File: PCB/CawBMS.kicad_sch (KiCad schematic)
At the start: 37 parts, among them CN1 SWD, CN2 I2C, CN3 SPI, CN4 USART, CN5 SWD, SW1 B3U-1000P, SW2 B3U-1000P, U1 STM32F103CBTx, U2 TCAN1044DRBRQ1, U5 CAN, X1 Crystal_16MHz_15pF_3P

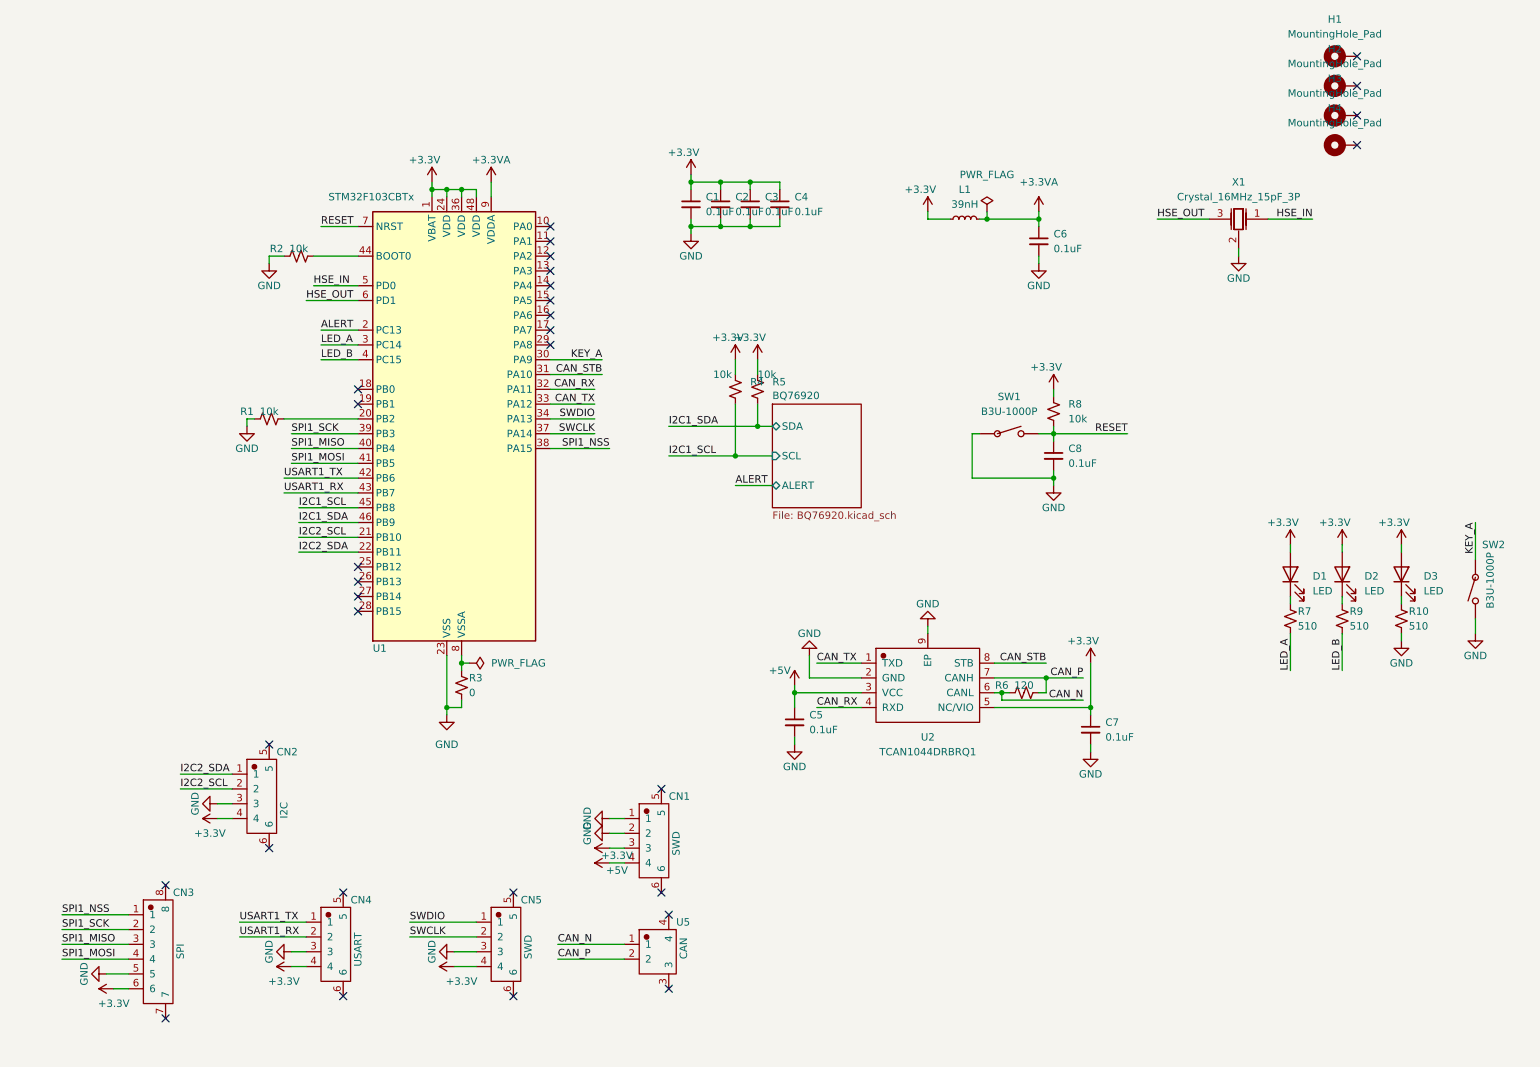
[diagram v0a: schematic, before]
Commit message: Signed-off-by: jasperThinkpad <2567434944@qq.com>
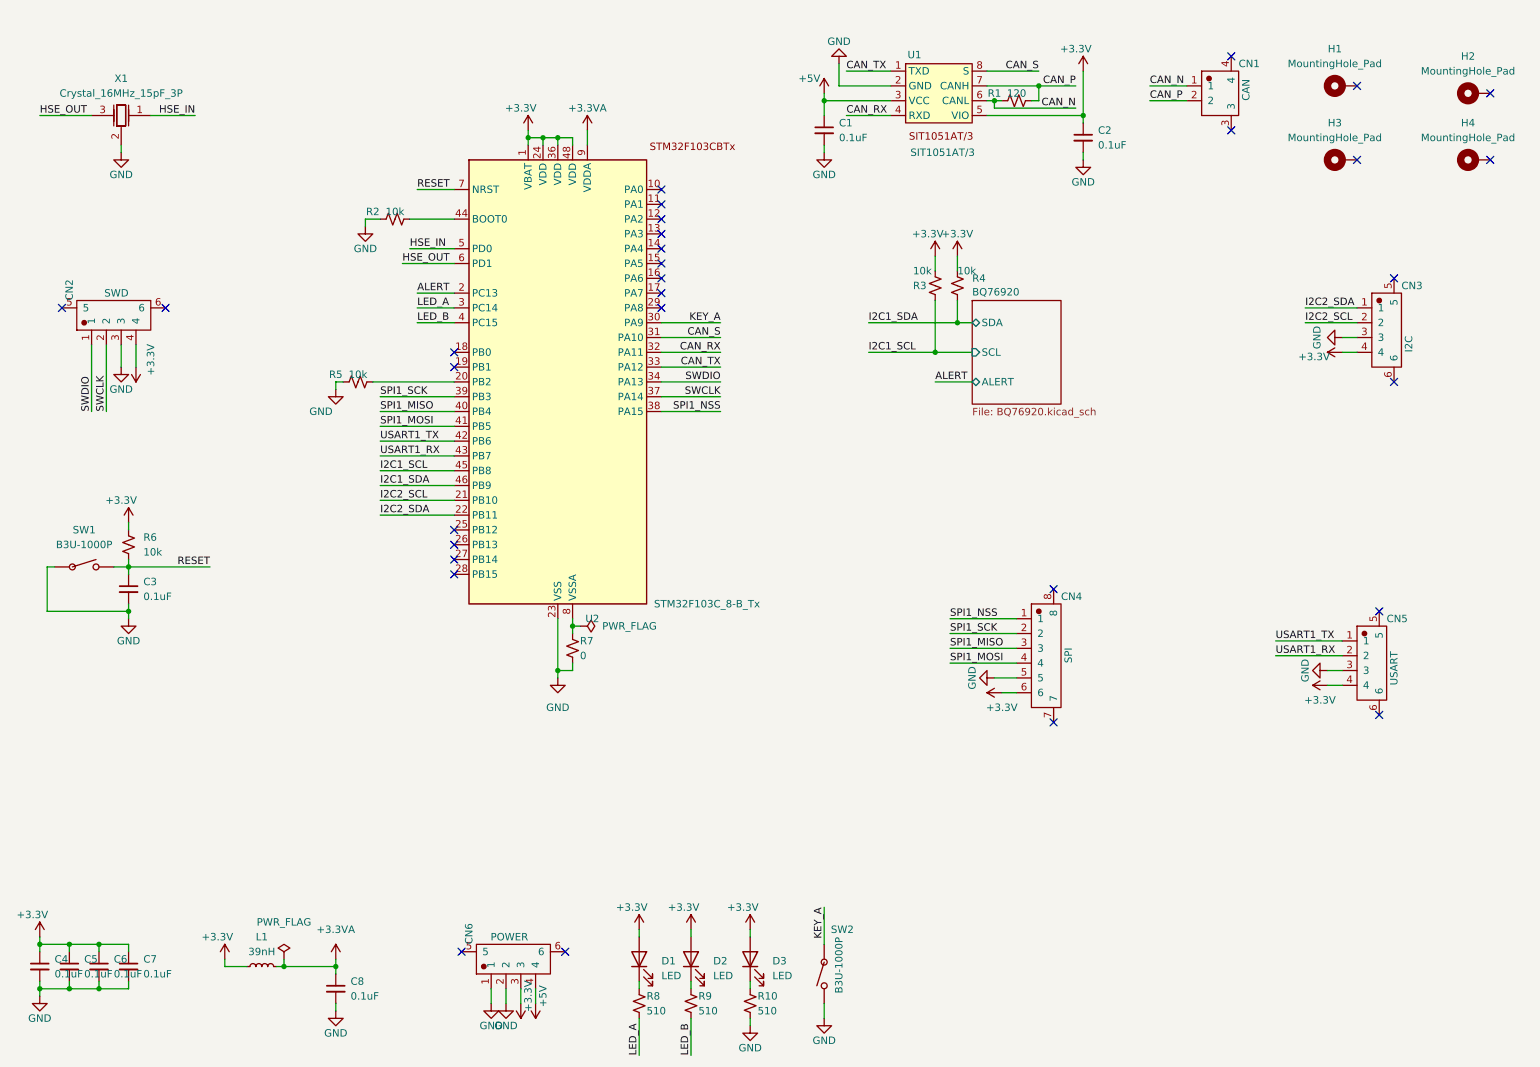
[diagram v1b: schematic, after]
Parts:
- removed U1: STM32F103CBTx, Package_QFP:LQFP-48_7x7mm_P0.5mm, symbol MCU_ST_STM32F1:STM32F103CBTx
- removed U2: TCAN1044DRBRQ1, Rick_CAN:TCAN1044DRBRQ1_DFN-8_L3.0-W3.0-P0.65-TL-EP2.4, symbol Rick_CAN:TCAN1044DRBRQ1
- added U1: SIT1051AT/3, Rick_CAN:ISO1044BDR_SOP-8, symbol bms:CAN
- added U2: STM32F103C_8-B_Tx, Package_QFP:LQFP-48_7x7mm_P0.5mm, symbol bms:STM32F103CBTx
- CN6: renamed from CN1; value SWD -> POWER
- renumbered C5 to C1, C7 to C2, C8 to C3, C1 to C4, C2 to C5, C3 to C6, C4 to C7, C6 to C8, U5 to CN1, CN5 to CN2, CN2 to CN3, CN3 to CN4, CN4 to CN5, R6 to R1, R4 to R3, R5 to R4, R1 to R5, R8 to R6, R3 to R7, R7 to R8
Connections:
- net +3.3V: now also U1.5 (VIO), U2.1 (VBAT), U2.24 (VDD), U2.36 (VDD), U2.48 (VDD)
- net +3.3VA: now also U2.9 (VDDA)
- net +5V: now also U1.3 (VCC)
- net ALERT: now also U2.2 (PC13)
- net CAN_N: now also U1.6 (CANL)
- net CAN_P: now also U1.7 (CANH)
- net CAN_RX: now also U1.4 (RXD), U2.32 (PA11)
- net CAN_TX: now also U1.1 (TXD), U2.33 (PA12)
- net GND: now also U1.2 (GND), U2.23 (VSS), U2.35 (VSS), U2.47 (VSS)
- net HSE_IN: now also U2.5 (PD0)
- net HSE_OUT: now also U2.6 (PD1)
- net I2C1_SCL: now also U2.45 (PB8)
- net I2C1_SDA: now also U2.46 (PB9)
- net I2C2_SCL: now also U2.21 (PB10)
- net I2C2_SDA: now also U2.22 (PB11)
- net KEY_A: now also U2.30 (PA9)
- net LED_A: now also U2.3 (PC14)
- net LED_B: now also U2.4 (PC15)
- net RESET: now also U2.7 (NRST)
- net SPI1_MISO: now also U2.40 (PB4)
- net SPI1_MOSI: now also U2.41 (PB5)
- net SPI1_NSS: now also U2.38 (PA15)
- net SPI1_SCK: now also U2.39 (PB3)
- net SWCLK: now also U2.37 (PA14)
- net SWDIO: now also U2.34 (PA13)
- net USART1_RX: now also U2.43 (PB7)
- net USART1_TX: now also U2.42 (PB6)
- net at R5.2: now also U2.20 (PB2)
- net at R7.1: now also U2.8 (VSSA)
- net at R2.2: now also U2.44 (BOOT0)
- new net CAN_S: U1.8 (S), U2.31 (PA10)
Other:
- moved on the sheet: C1, C2, C3, C4, C5, C6, C7, C8, CN1, CN2, CN3, CN4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
